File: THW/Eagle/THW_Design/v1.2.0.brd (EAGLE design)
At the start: 100 x 200 mm, 20 parts

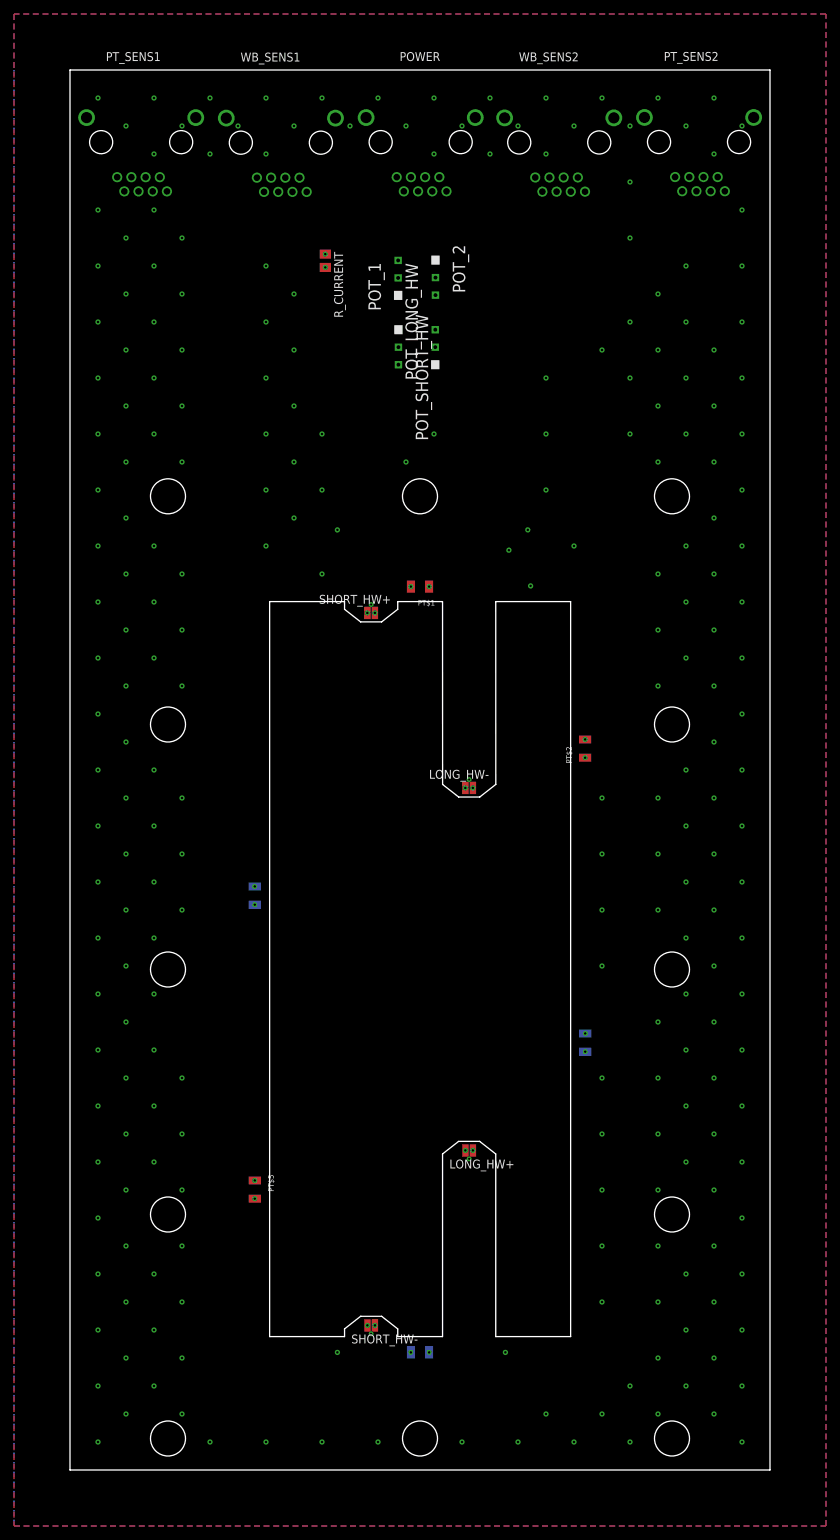
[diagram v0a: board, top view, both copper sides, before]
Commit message: Minor changes to design and logo package
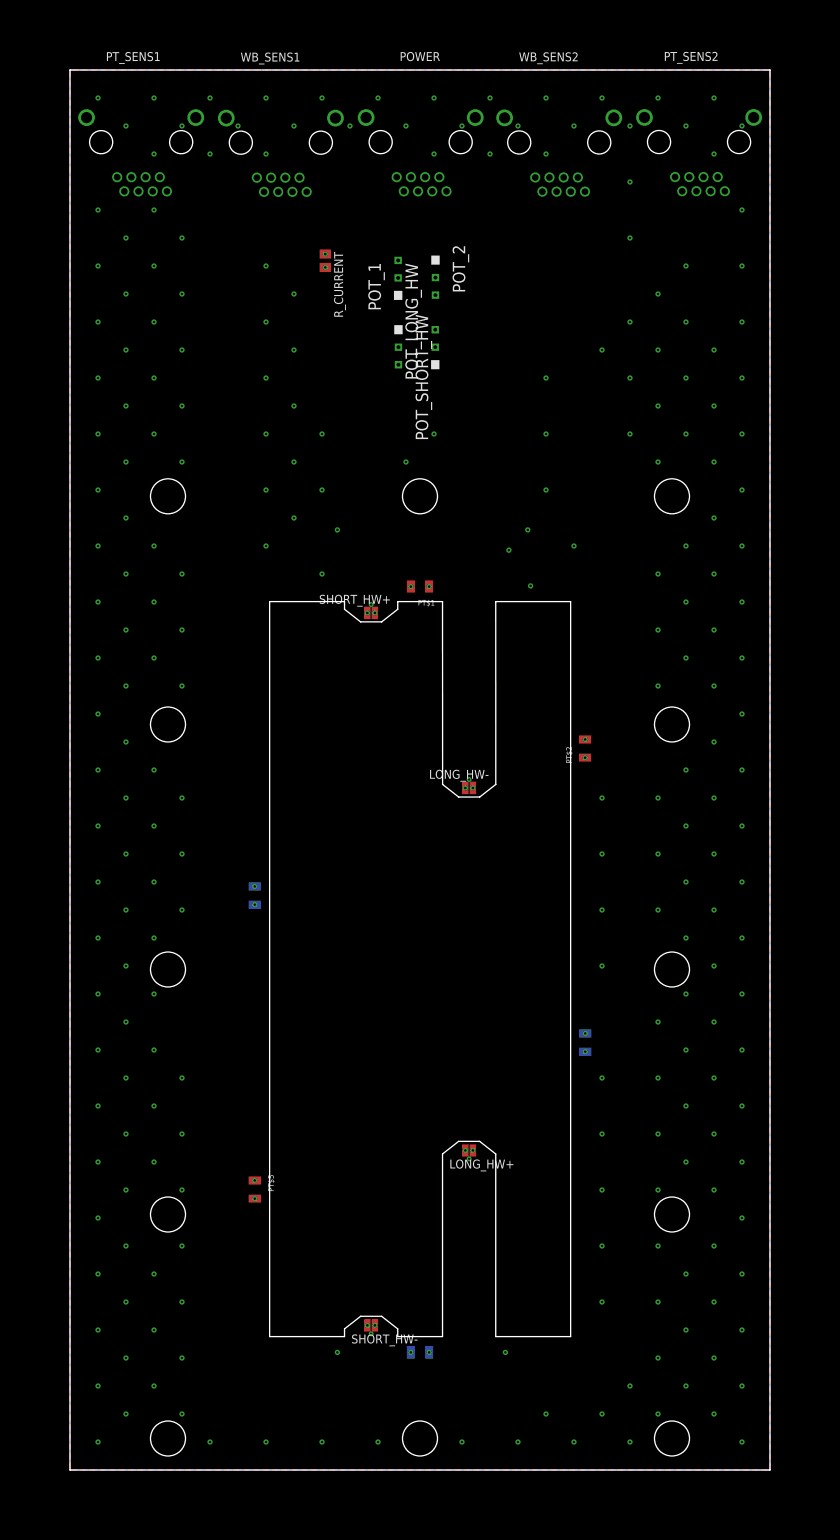
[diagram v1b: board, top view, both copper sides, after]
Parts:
- added U$1: (no value), AD_LOGO:AD_LOGO
